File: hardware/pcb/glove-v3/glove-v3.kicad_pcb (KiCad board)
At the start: 2 copper layers, 19 parts, among them U1 XIAO-ESP32C3, U2 CD74HC4067M96

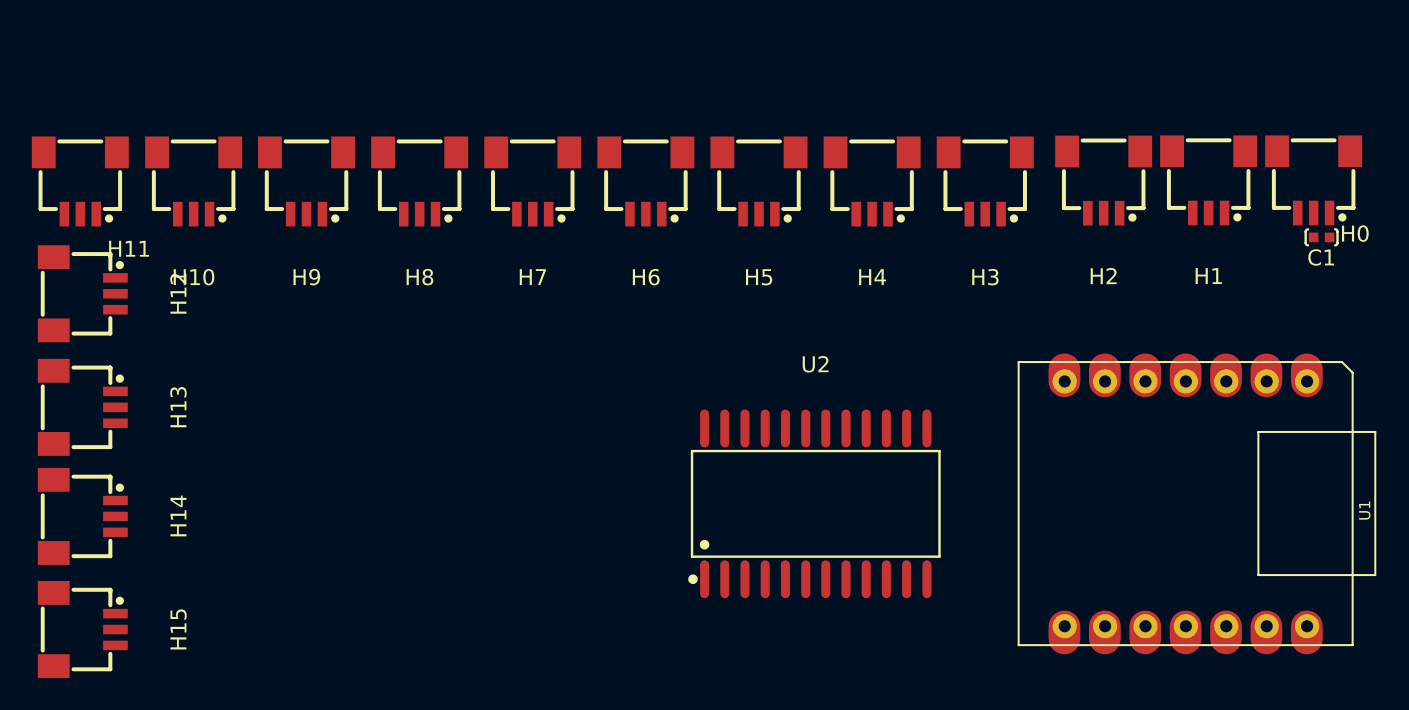
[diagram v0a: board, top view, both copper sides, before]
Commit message: schematic done and board layout done
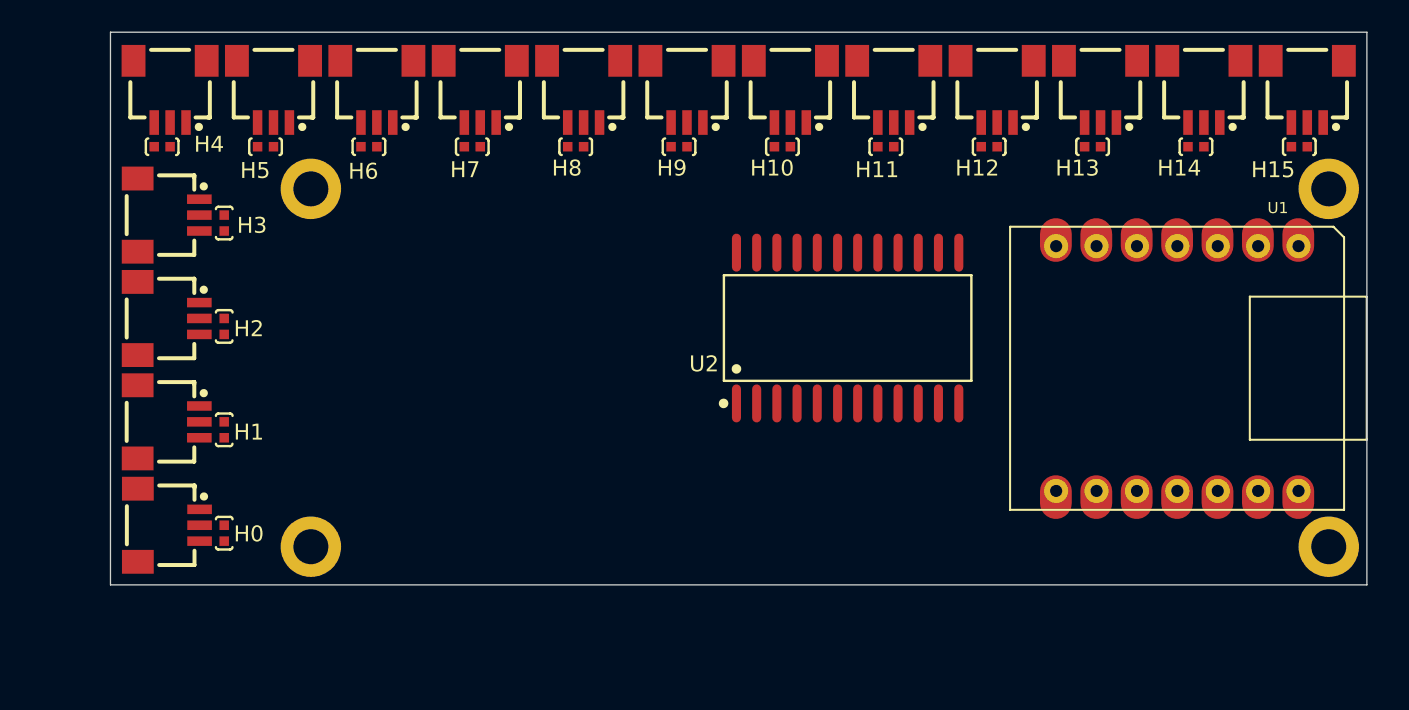
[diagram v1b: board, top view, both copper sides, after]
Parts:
- added C0: C-0402-0.01uF, 0_easyeda2kicad:C0402, F.Cu at (108.6, 56.2)
- added C10: C-0402-0.01uF, 0_easyeda2kicad:C0402, F.Cu at (143.7, 31.9)
- added C11: C-0402-0.01uF, 0_easyeda2kicad:C0402, F.Cu at (150.2, 31.9)
- added C12: C-0402-0.01uF, 0_easyeda2kicad:C0402, F.Cu at (156.7, 31.9)
- added C13: C-0402-0.01uF, 0_easyeda2kicad:C0402, F.Cu at (163.2, 31.9)
- added C14: C-0402-0.01uF, 0_easyeda2kicad:C0402, F.Cu at (169.7, 31.9)
- added C15: C-0402-0.01uF, 0_easyeda2kicad:C0402, F.Cu at (176.2, 31.9)
- added C2: C-0402-0.01uF, 0_easyeda2kicad:C0402, F.Cu at (108.6, 43.2)
- added C3: C-0402-0.01uF, 0_easyeda2kicad:C0402, F.Cu at (108.6, 36.7)
- added C4: C-0402-0.01uF, 0_easyeda2kicad:C0402, F.Cu at (104.7, 31.9)
- added C5: C-0402-0.01uF, 0_easyeda2kicad:C0402, F.Cu at (111.2, 31.9)
- added C6: C-0402-0.01uF, 0_easyeda2kicad:C0402, F.Cu at (117.7, 31.9)
- added C7: C-0402-0.01uF, 0_easyeda2kicad:C0402, F.Cu at (124.2, 31.9)
- added C8: C-0402-0.01uF, 0_easyeda2kicad:C0402, F.Cu at (130.7, 31.9)
- added C9: C-0402-0.01uF, 0_easyeda2kicad:C0402, F.Cu at (137.2, 31.9)
- added REF**: MountingHole_2.2mm_M2_DIN965_Pad, 0_MountingHole:MountingHole_2.2mm_M2_DIN965_Pad, F.Cu at (114.0, 34.5)
- added REF**: MountingHole_2.2mm_M2_DIN965_Pad, 0_MountingHole:MountingHole_2.2mm_M2_DIN965_Pad, F.Cu at (178.1, 57.0)
- added REF**: MountingHole_2.2mm_M2_DIN965_Pad, 0_MountingHole:MountingHole_2.2mm_M2_DIN965_Pad, F.Cu at (114.0, 57.0)
- added REF**: MountingHole_2.2mm_M2_DIN965_Pad, 0_MountingHole:MountingHole_2.2mm_M2_DIN965_Pad, F.Cu at (178.1, 34.5)
- moved H15 84.0 mm to (176.7, 28.4), turned to 180 degrees
- moved H14 75.3 mm to (170.2, 28.4), turned to 180 degrees
- moved H0 75.2 mm to (105.1, 55.7), turned to -90 degrees
- moved C1 70.1 mm to (108.6, 49.7), turned to -90 degrees
- moved H1 67.1 mm to (105.1, 49.2), turned to -90 degrees
- moved H13 66.9 mm to (163.7, 28.4), turned to 180 degrees
- moved H2 59.4 mm to (105.1, 42.7), turned to -90 degrees
- moved H12 58.8 mm to (157.2, 28.4), turned to 180 degrees
- moved H11 51.5 mm to (150.7, 28.4)
- moved H3 51.4 mm to (105.1, 36.2), turned to -90 degrees
- moved H4 44.5 mm to (105.2, 28.4)
- moved H10 38.0 mm to (144.2, 28.4)
- moved H5 31.1 mm to (111.7, 28.4)
- moved H9 24.6 mm to (137.7, 28.4)
- moved H6 17.9 mm to (118.2, 28.4)
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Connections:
- H0 pad 1: +3V3 -> /HALL_0
- H0 pad 3: /HALL_0 -> +3V3
- H1 pad 1: +3V3 -> /HALL_1
- H1 pad 3: /HALL_0 -> +3V3
- H10 pad 1: +3V3 -> /HALL_10
- H10 pad 3: /HALL_0 -> +3V3
- H11 pad 1: +3V3 -> /HALL_11
- H11 pad 3: /HALL_0 -> +3V3
- H12 pad 1: +3V3 -> /HALL_12
- H12 pad 3: /HALL_0 -> +3V3
- H13 pad 1: +3V3 -> /HALL_13
- H13 pad 3: /HALL_0 -> +3V3
- H14 pad 1: +3V3 -> /HALL_14
- H14 pad 3: /HALL_0 -> +3V3
- H15 pad 1: +3V3 -> /HALL_15
- H15 pad 3: /HALL_0 -> +3V3
- H2 pad 1: +3V3 -> /HALL_2
- H2 pad 3: /HALL_0 -> +3V3
- H3 pad 1: +3V3 -> /HALL_3
- H3 pad 3: /HALL_0 -> +3V3
- H4 pad 1: +3V3 -> /HALL_4
- H4 pad 3: /HALL_0 -> +3V3
- H5 pad 1: +3V3 -> /HALL_5
- H5 pad 3: /HALL_0 -> +3V3
- H6 pad 1: +3V3 -> /HALL_6
- H6 pad 3: /HALL_0 -> +3V3
- H7 pad 1: +3V3 -> /HALL_7
- H7 pad 3: /HALL_0 -> +3V3
- H8 pad 1: +3V3 -> /HALL_8
- H8 pad 3: /HALL_0 -> +3V3
- H9 pad 1: +3V3 -> /HALL_9
- H9 pad 3: /HALL_0 -> +3V3
- U1 pad 10: unconnected-(U1-PA5_A9_D9_MISO-Pad10) -> /S0
- U1 pad 12: unconnected-(U1-3V3-Pad12) -> +3V3
- U1 pad 13: unconnected-(U1-GND-Pad13) -> GND
- U1 pad 3: unconnected-(U1-PA10_A2_D2-Pad3) -> /MUX_OUT
- U1 pad 5: unconnected-(U1-PA8_A4_D4_SDA-Pad5) -> /S2
- U1 pad 6: unconnected-(U1-PA9_A5_D5_SCL-Pad6) -> /S3
- U1 pad 9: unconnected-(U1-PA7_A8_D8_SCK-Pad9) -> /S1
- U2 pad 1: unconnected-(U2-COMMONINPUT/OUTPUT-Pad1) -> /MUX_OUT
- U2 pad 10: unconnected-(U2-S0-Pad10) -> /S0
- U2 pad 11: unconnected-(U2-S1-Pad11) -> /S1
- U2 pad 12: unconnected-(U2-GND-Pad12) -> GND
- U2 pad 13: unconnected-(U2-S3-Pad13) -> /S3
- U2 pad 14: unconnected-(U2-S2-Pad14) -> /S2
- U2 pad 15: unconnected-(U2-~{E}-Pad15) -> GND
- U2 pad 16: unconnected-(U2-I15-Pad16) -> /HALL_15
- U2 pad 17: unconnected-(U2-I14-Pad17) -> /HALL_14
- U2 pad 18: unconnected-(U2-I13-Pad18) -> /HALL_13
- U2 pad 19: unconnected-(U2-I12-Pad19) -> /HALL_12
- U2 pad 2: unconnected-(U2-I7-Pad2) -> /HALL_7
- U2 pad 20: unconnected-(U2-I11-Pad20) -> /HALL_11
- U2 pad 21: unconnected-(U2-I10-Pad21) -> /HALL_10
- U2 pad 22: unconnected-(U2-I9-Pad22) -> /HALL_9
- U2 pad 23: unconnected-(U2-I8-Pad23) -> /HALL_8
- U2 pad 24: unconnected-(U2-VCC-Pad24) -> +3V3
- U2 pad 3: unconnected-(U2-I6-Pad3) -> /HALL_6
- U2 pad 4: unconnected-(U2-I5-Pad4) -> /HALL_5
- U2 pad 5: unconnected-(U2-I4-Pad5) -> /HALL_4
- U2 pad 6: unconnected-(U2-I3-Pad6) -> /HALL_3
- U2 pad 7: unconnected-(U2-I2-Pad7) -> /HALL_2
- U2 pad 8: unconnected-(U2-I1-Pad8) -> /HALL_1
- U2 pad 9: unconnected-(U2-I0-Pad9) -> /HALL_0
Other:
- board outline added: 79 x 34.8 mm
- copper layers 2 -> 4
